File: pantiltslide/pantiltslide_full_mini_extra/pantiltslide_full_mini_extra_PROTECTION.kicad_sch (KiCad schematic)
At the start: 81 parts, among them J1 Conn_01x22_Socket, J17 Motor_Slide, J18 Motor_Pan, J19 Motor_Tilt, J2 Conn_01x22_Socket, J20 TCA9548A_Mux, J21 AS5600_Pan, J22 AS5600_Tilt, J23 OLED, J24 TCA9548A_Mux, J26 Limit_Min, J27 Limit_Max, J28 Motor_Aux, J29 Enc_Slide, J3 MUX_2, J30 Enc_Pan, J31 Enc_Tilt, J32 Enc_Aux, J33 Btn_SetKeyframe, J34 Btn_ClearKeyframe, J35 Btn_PlayPause, J36 Btn_Reset, J37 5V_In, J38 24V_In, J4 MUX_3, J41 Aux_Max, J5 MUX_4, J6 MUX_5, J7 MUX_6, J8 MUX_7, U1 tmc2209, U2 tmc2209, U3 tmc2209, U4 tmc2209

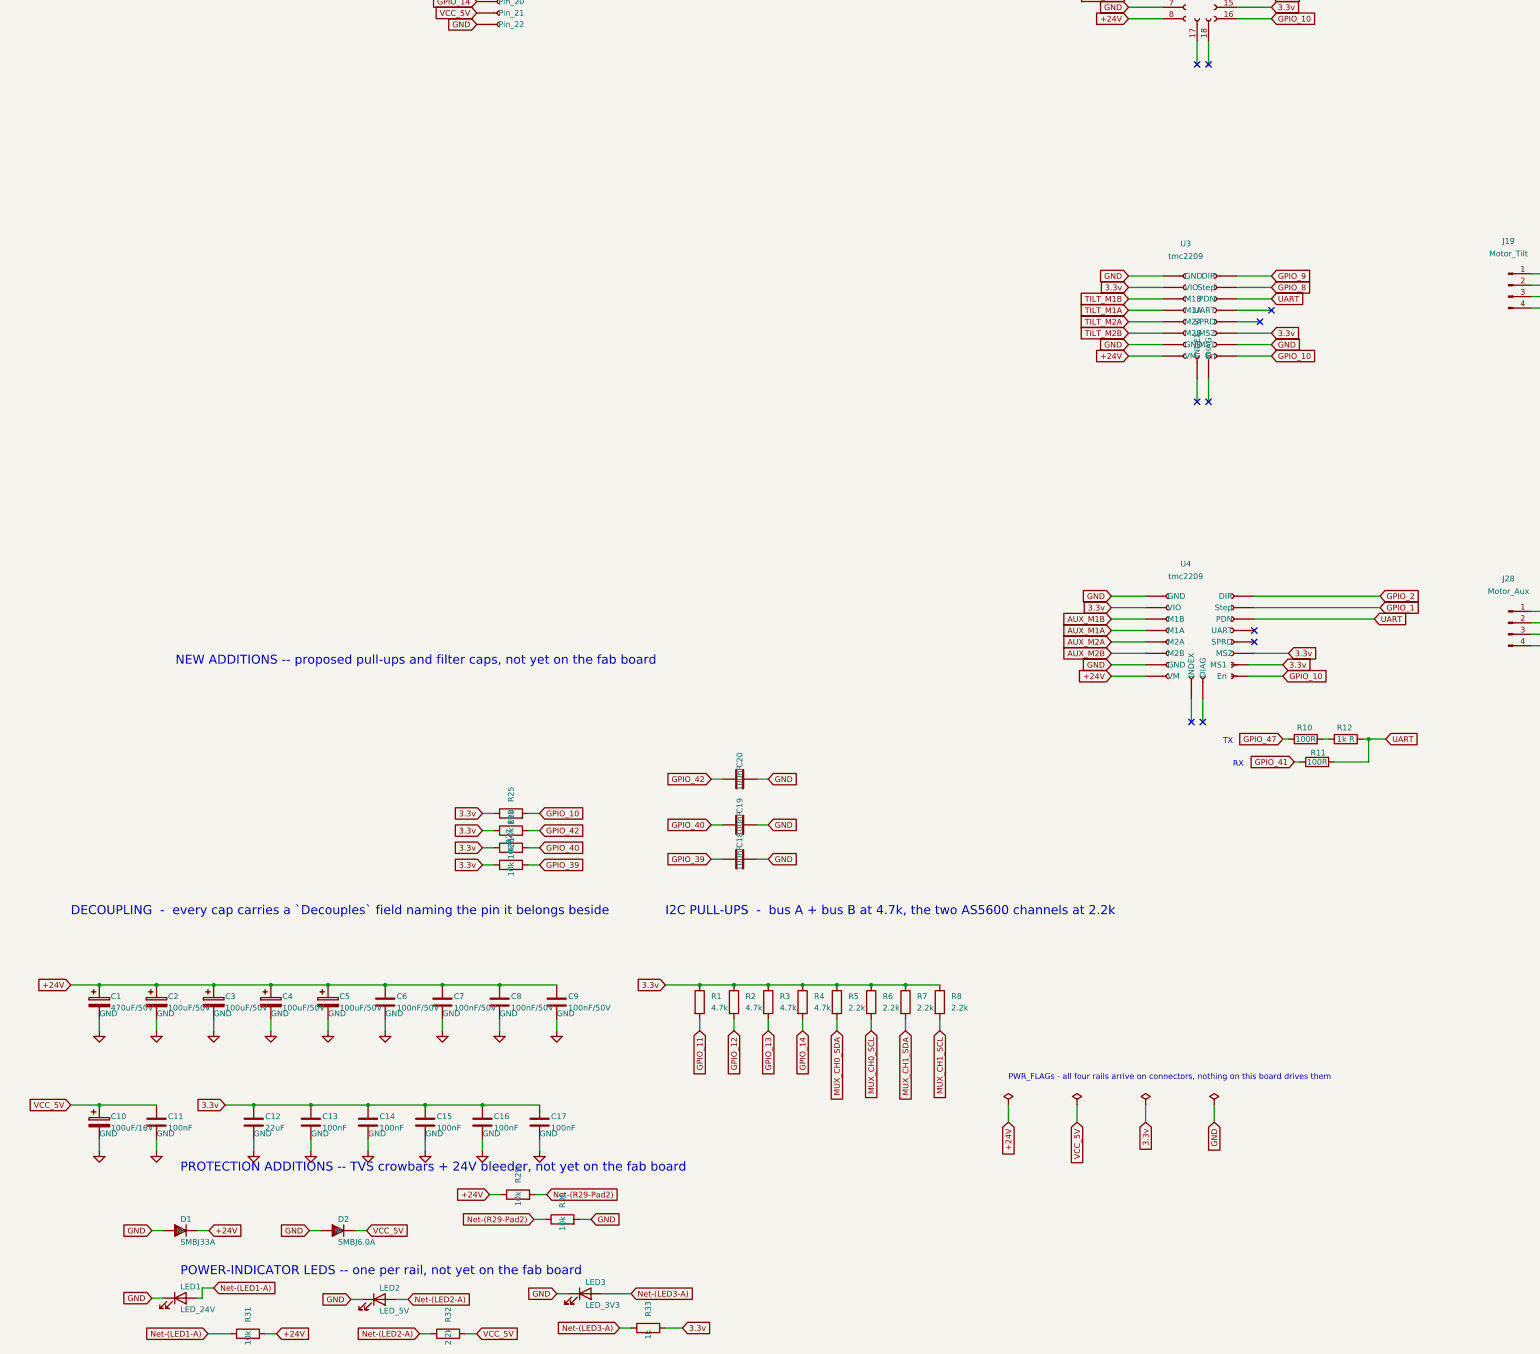
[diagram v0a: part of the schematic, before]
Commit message: formatting
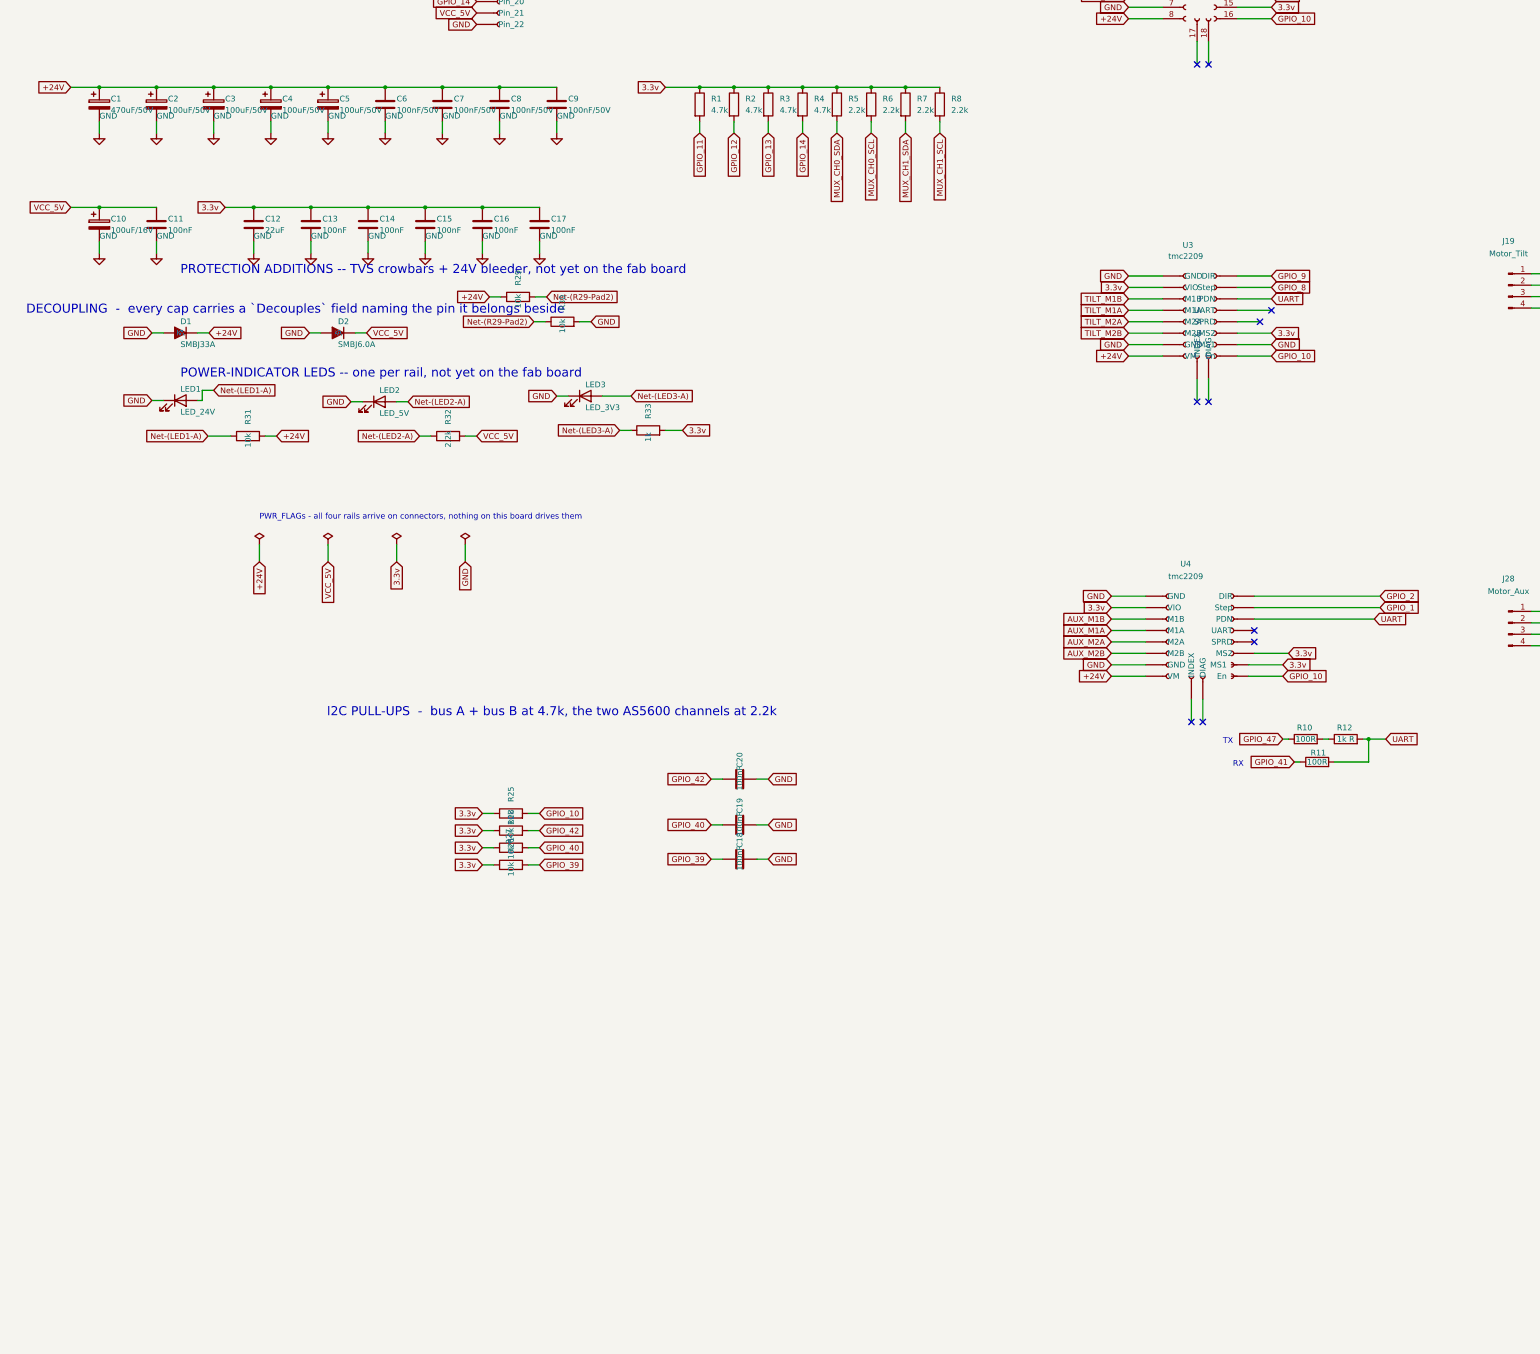
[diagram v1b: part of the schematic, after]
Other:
- note removed: "NEW ADDITIONS -- proposed pull-ups and filter caps, not yet on the fab board"
- moved on the sheet: C1, C10, C11, C12, C13, C14, C15, C16, C17, C2, C3, C4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
